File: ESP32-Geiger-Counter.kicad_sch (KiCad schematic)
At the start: 79 parts, among them J1 2s1p Lipo Battery Pack (8.4V-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, J2 USB_C_Receptacle_USB2.0_16P, J3 SBM20 +, J4 SBM20 -, J5 Conn_01x07, Q1 Q_NMOS_GDS, Q2 2N3904, Q3 2N7002, SW1 SW_SPDT, SW2 RESET, SW3 BOOT, U1 BQ25886RGE, U2 AP63203WU, U3 ESP32-S3-WROOM-1, U4 UCC27517DBVR, U5 USBLC6-2SC6

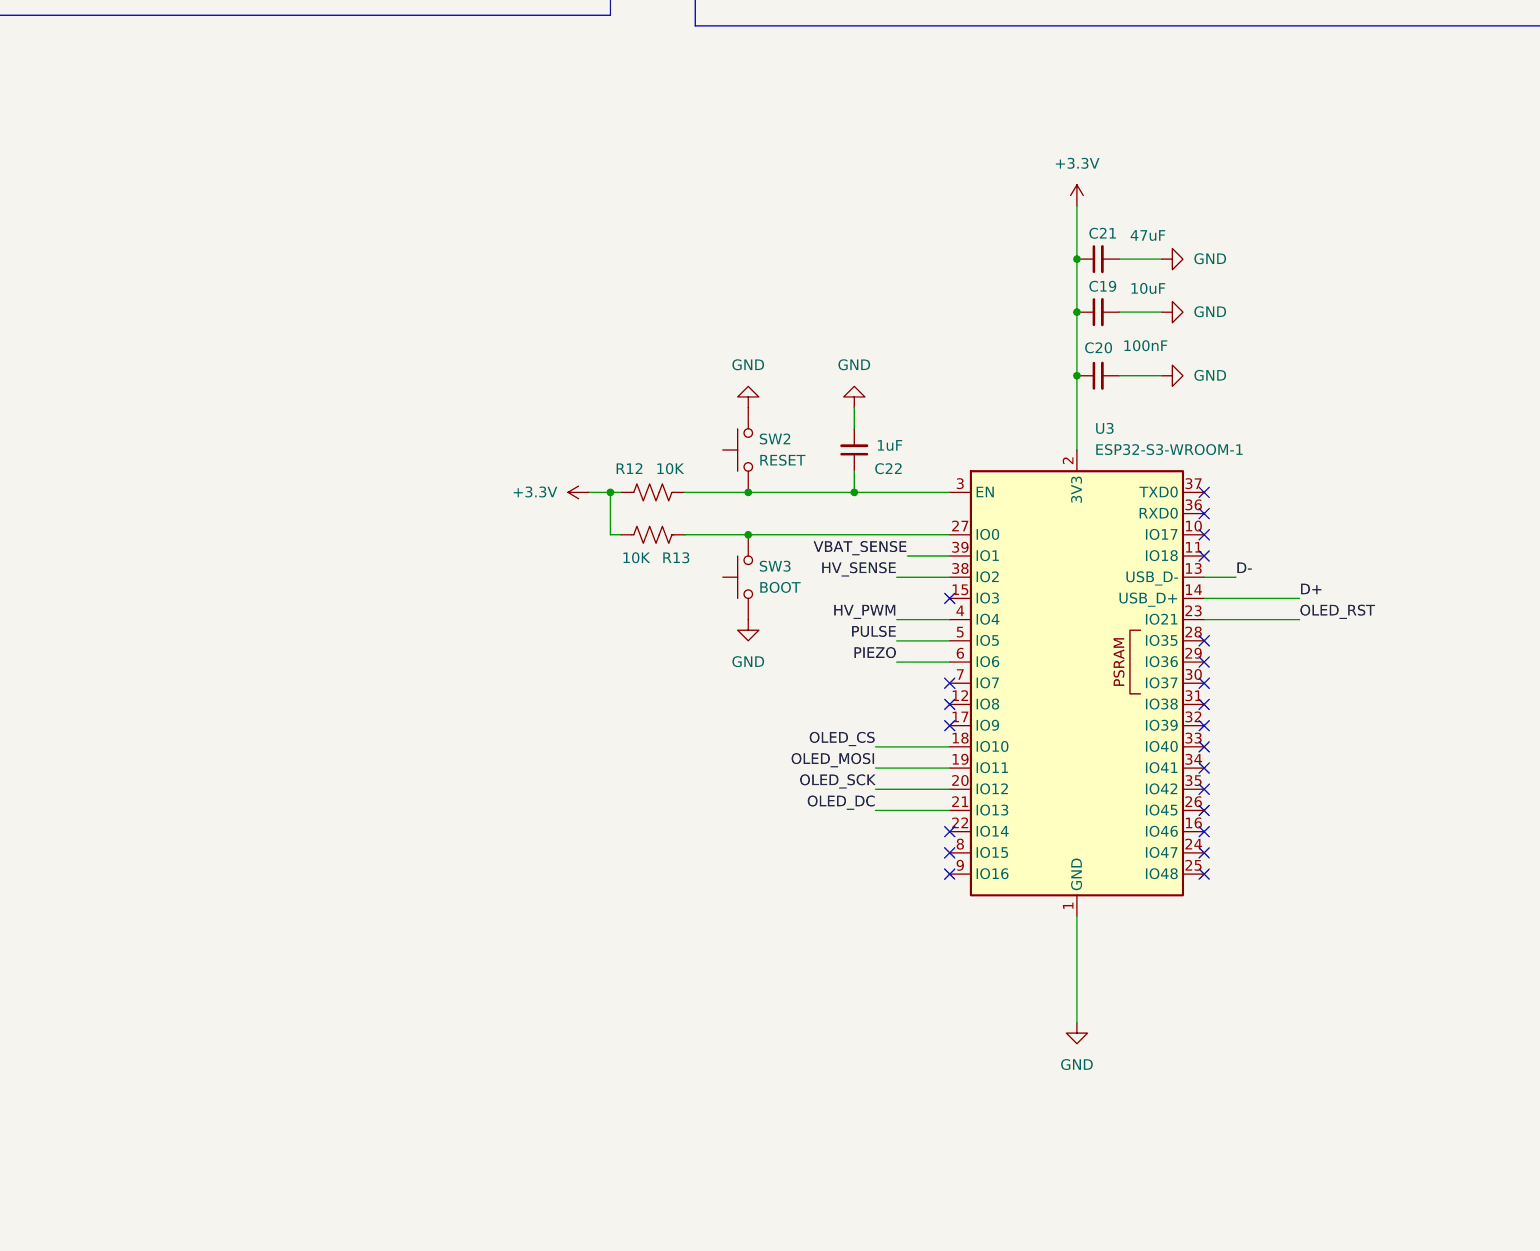
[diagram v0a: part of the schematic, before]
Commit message: added a bunch of passive footprints
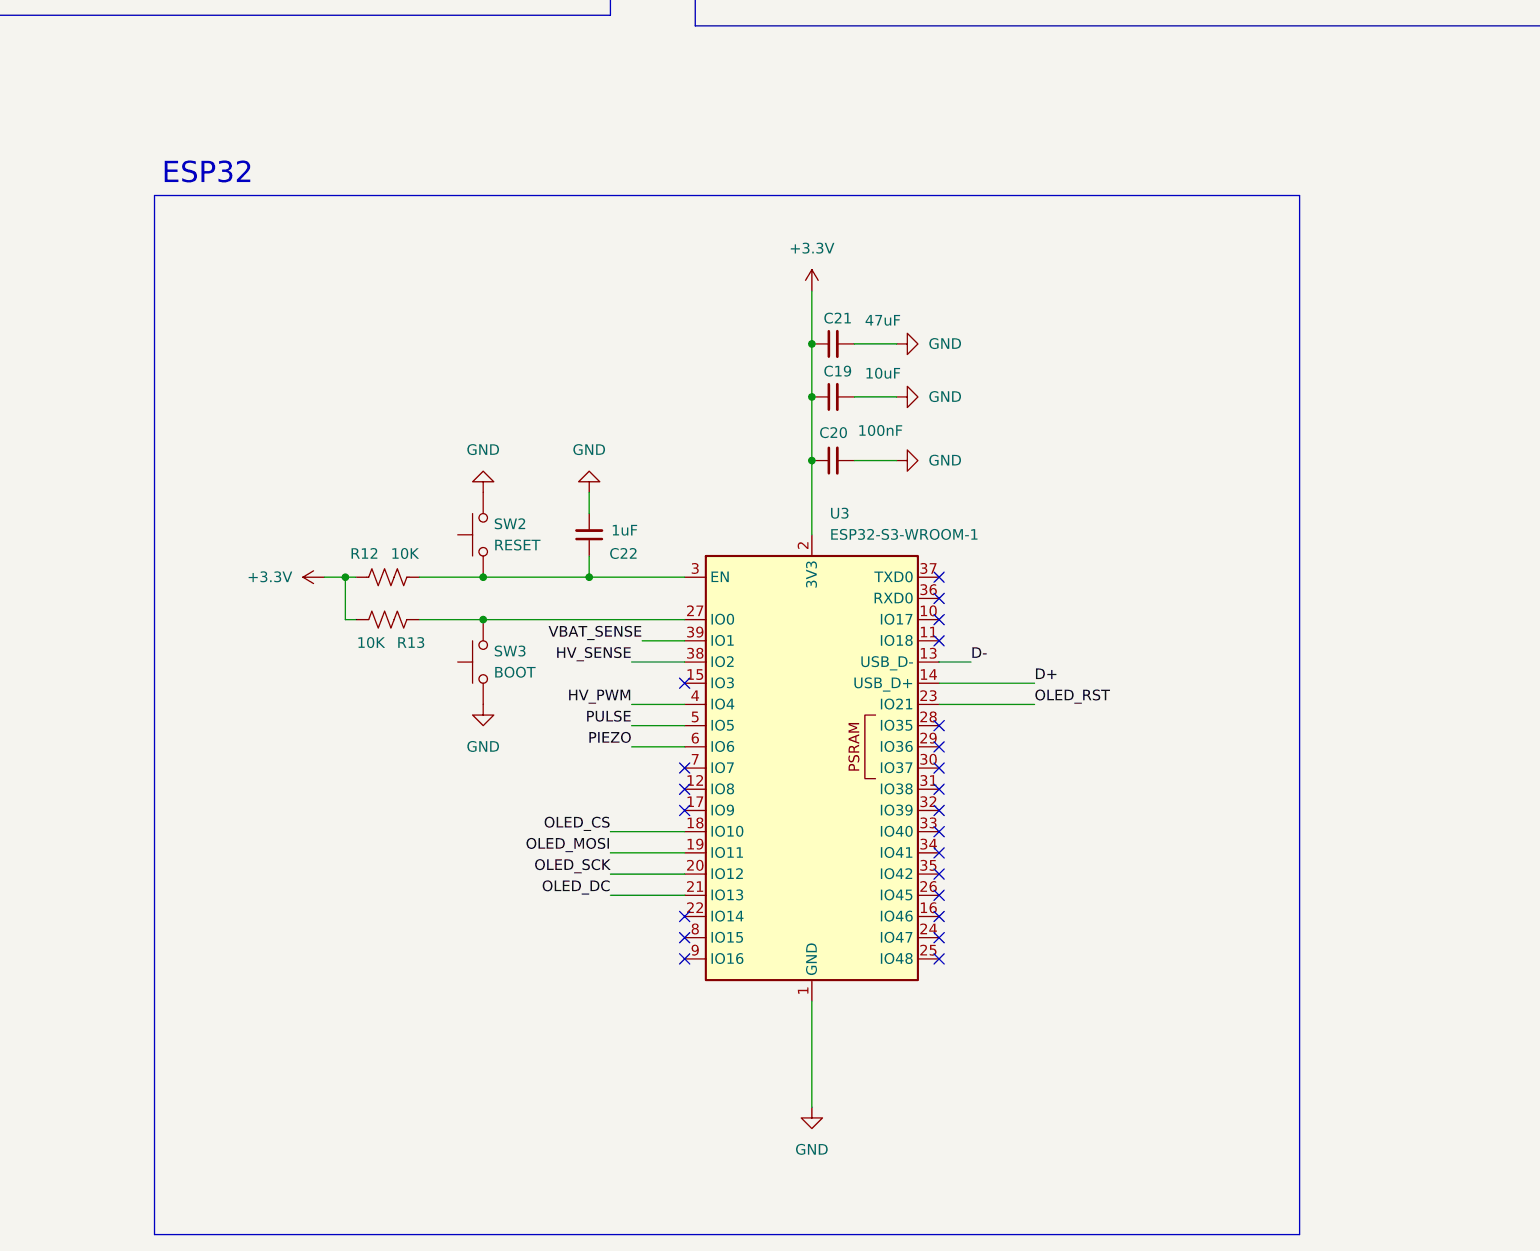
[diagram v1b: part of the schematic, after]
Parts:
- C14, C17, C18, C26, C28, C29, C31: footprint (none) -> Capacitor_SMD:C_0805_2012Metric
- C15, C16, C23, C24, C25, C27, C30: footprint (none) -> Capacitor_SMD:C_1206_3216Metric
- D3, D4, D5, D6: footprint (none) -> Diode_SMD:D_SMA
- F1: footprint (none) -> Fuse:Fuse_2920_7451Metric
- R1, R10, R11, R17, R2, R20, R21, R22, R23, R24, R25, R26, R27: footprint (none) -> Resistor_SMD:R_0805_2012Metric
- R14, R15, R16: footprint (none) -> Resistor_SMD:R_1206_3216Metric
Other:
- note added: "ESP32"
- moved on the sheet: C19, C20, C21, C22, R12, R13, SW2, SW3, U3
